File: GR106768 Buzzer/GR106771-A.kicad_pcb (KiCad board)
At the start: 4 copper layers, 76 x 58 mm, 348 parts, among them IC1 L-BC-SOT23-5, IC2 L-BC-SO08, IC3 L-BC-SO08, IC4 L-BC-SOT23-5, IC5 L-BC-SO08, IC6 L-BC-SO08, IC7 L-BC-SOT23-6, IC8 L-BC-DFN10, IC9 L-BC-SOT23-6, J1 BAR-10-1007, J2 MIRECMS, J3 MIRECMS, SW1 SI-10-NK236, T1 Q-BC-SOT23-BEC, T10 Q-BC-SOT23-GSD, T11 Q-BC-SOT23-GSD, T12 Q-BC-SOT23-GSD, T13 Q-BC-SOT23-GSD, T2 Q-BC-SOT23-BEC, T3 Q-BC-SOT23-BEC, T4 Q-BC-SOT23-BEC, T5 Q-BC-SOT23-GSD, T6 Q-BC-SOT23-GSD, T7 Q-BC-SOT23-GSD, T8 Q-BC-SOT23-GSD, T9 Q-BC-SOT23-GSD

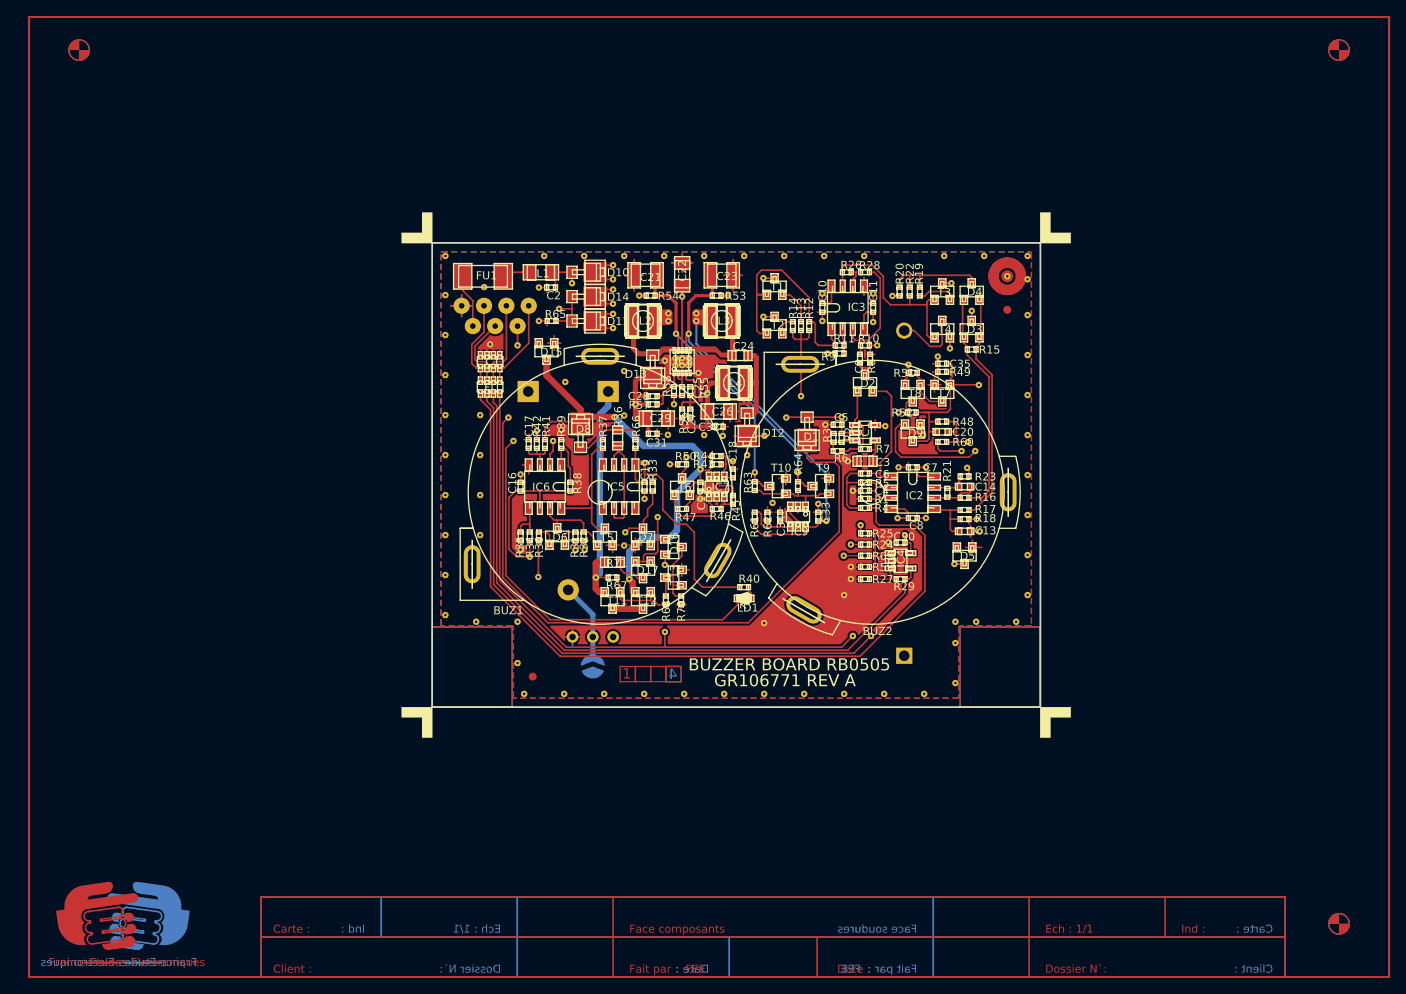
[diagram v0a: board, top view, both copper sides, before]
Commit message: Update holes 4
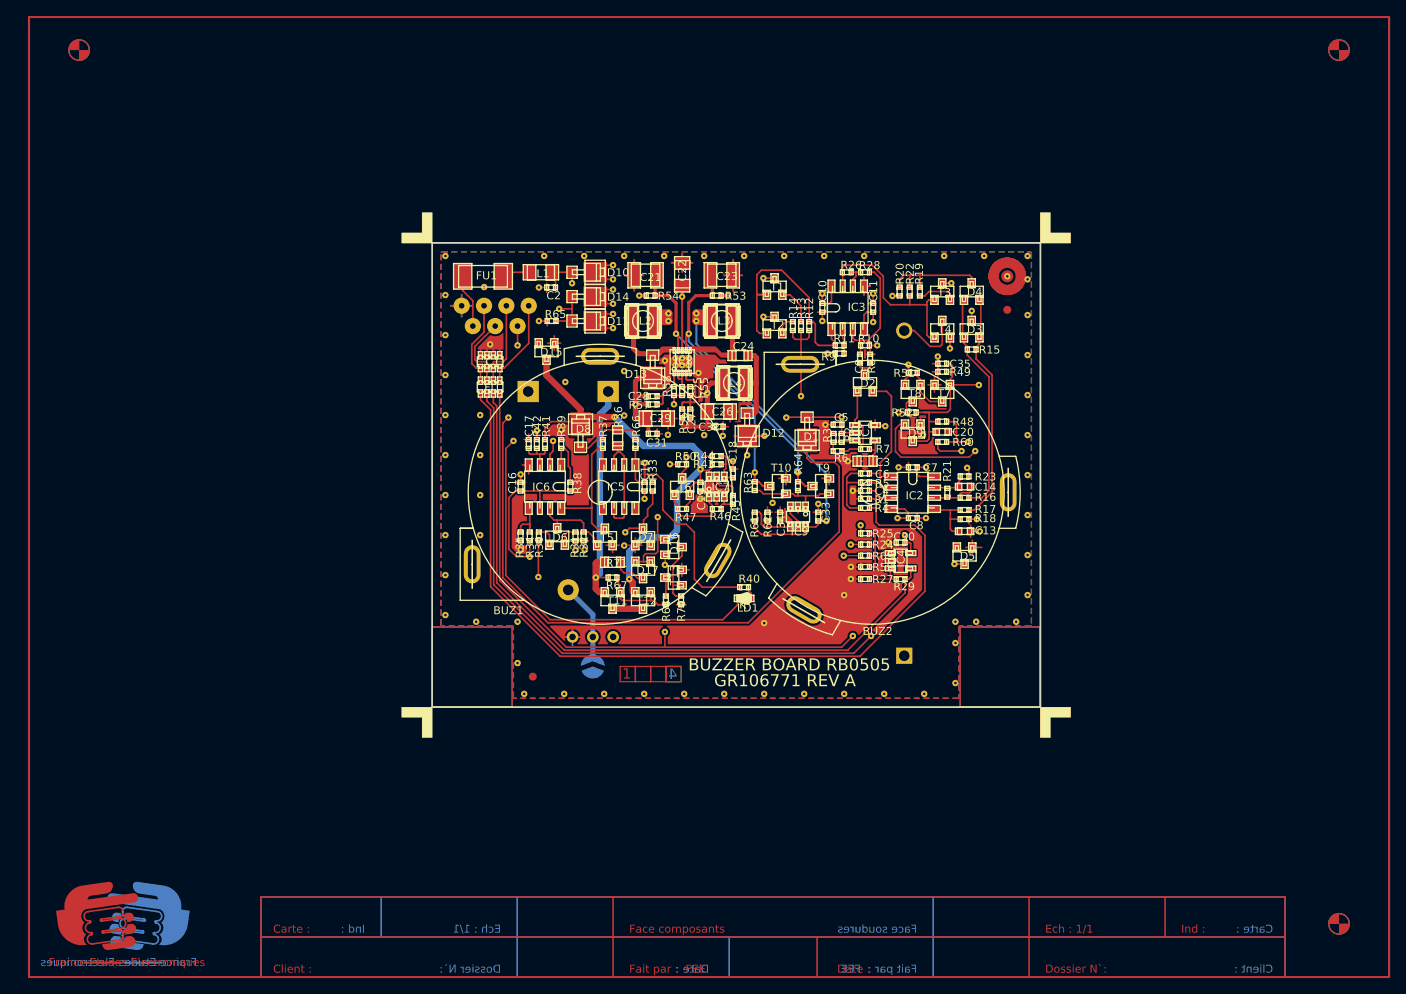
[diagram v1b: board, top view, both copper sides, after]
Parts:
- removed the V171 at (51.4, -18.9)
- added R8: R-BC-R0402, R0402, F.Cu at (54.7, -43.6)
- V171: renamed from R8; value R-BC-R0402 -> VIA-08X03_1011; footprint R0402 -> VIA-08X03_1011
- moved V171 24.9 mm to (51.4, -18.9), turned to 0 degrees
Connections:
- net /VBAT renamed VBAT
- net SUPPLY-BUZ renamed /SUPPLY-BUZ
- C19 pad 1: VCHARG -> /VCHARG
- D15 pad 3: VCHARG -> /VCHARG
- D8 pad K: VCHARG -> /VCHARG
- IC7 pad 6: VCHARG -> /VCHARG
- R41 pad 1: VCHARG -> /VCHARG
- R43 pad 2: VCHARG -> /VCHARG
- R47 pad 2: VCHARG -> /VCHARG
- R69 pad 1: VCHARG -> /VCHARG
- T12 pad S: VCHARG -> /VCHARG
- T6 pad S: VCHARG -> /VCHARG
- V165 pad ~: VCHARG -> /VCHARG
- V173 pad ~: VCHARG -> /VCHARG
- V49 pad ~: VCHARG -> /VCHARG
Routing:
- net VCHARG: track 98.1 -> 0.00 mm
- net /VCHARG: track 0.00 -> 98.1 mm
